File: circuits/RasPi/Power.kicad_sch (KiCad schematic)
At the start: 84 parts, among them J4 Conn_01x02_Pin, Q11 2N7002, Q12 SSM6J808R, Q14 SSM6J808R, Q15 S8550, Q16 SSM6J808R, Q17 S8550, Q6 SSM3J332R, Q7 S8550, Q8 SSM3J332R, Q9 S8550, SW4 SW_SPDT, U13 TPS54560BDDA, U16 AZ1117CH-3.3, U17 M51957B, U19 DCDC_TPS61023

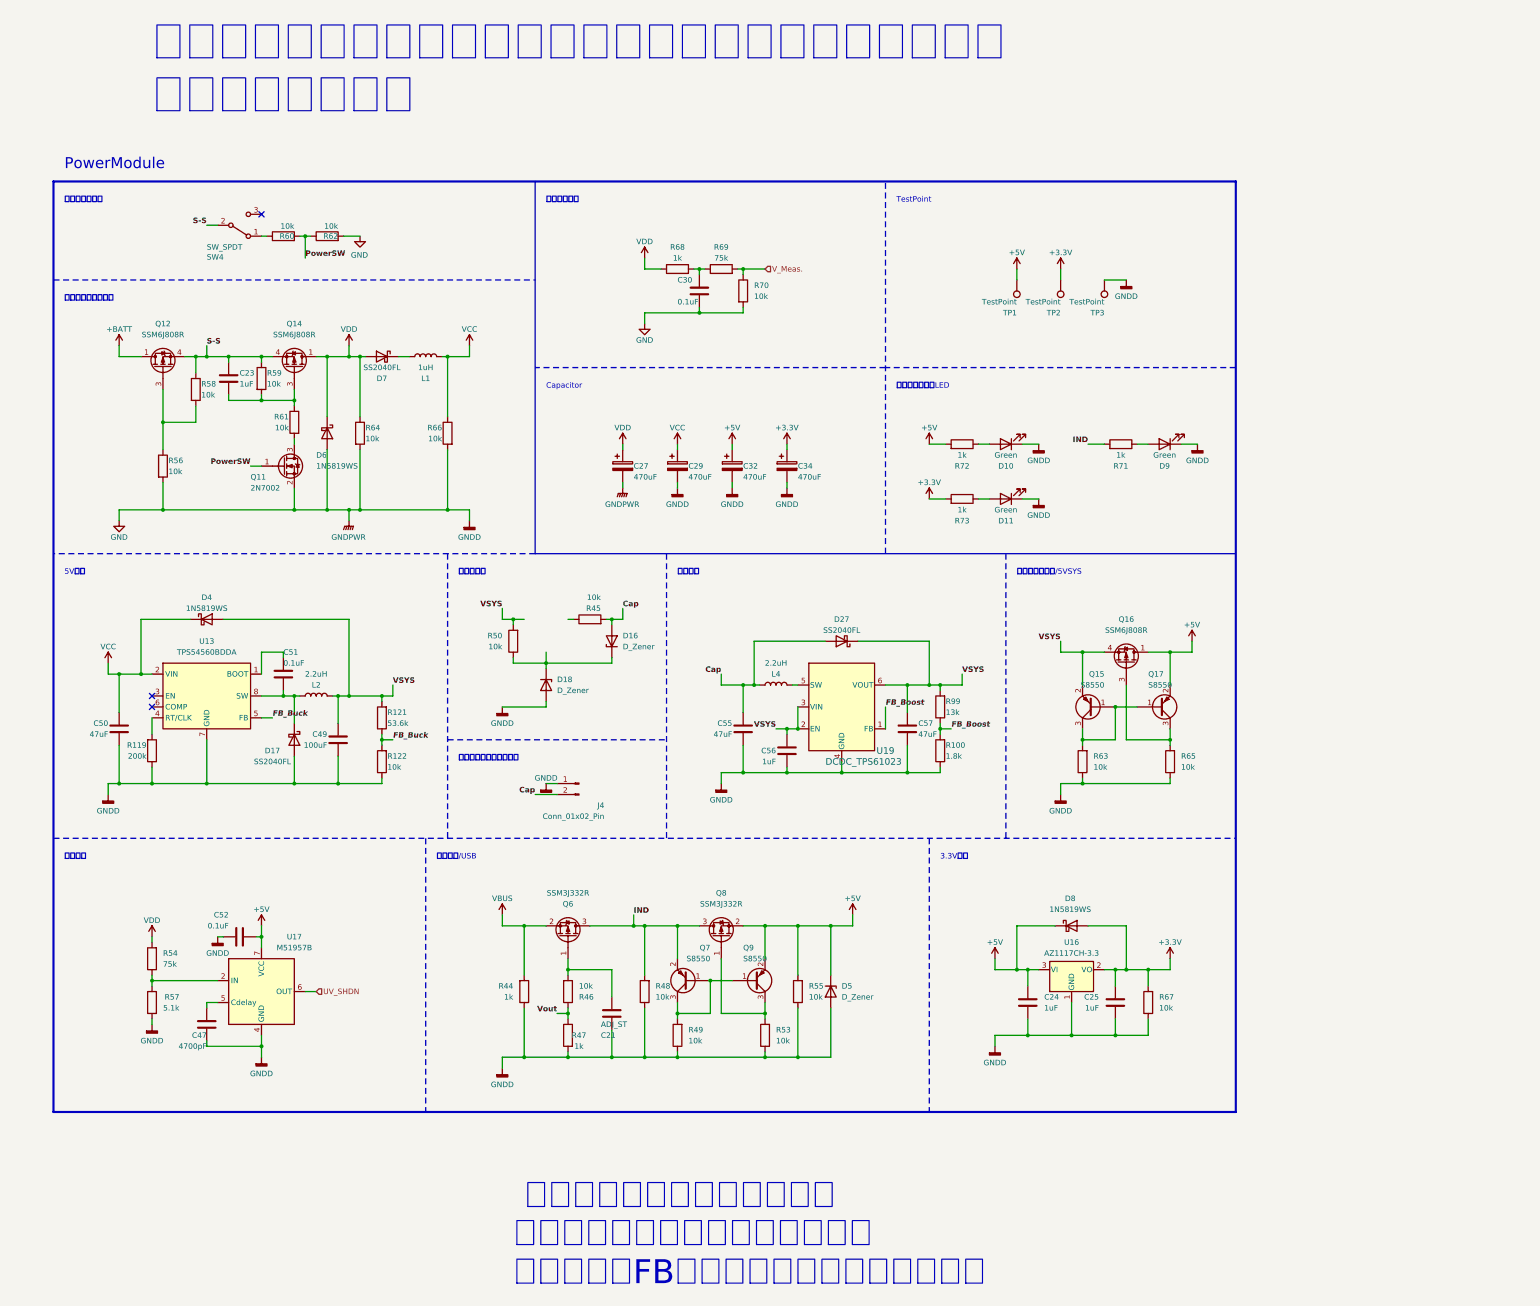
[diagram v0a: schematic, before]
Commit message: raspi基板回路図
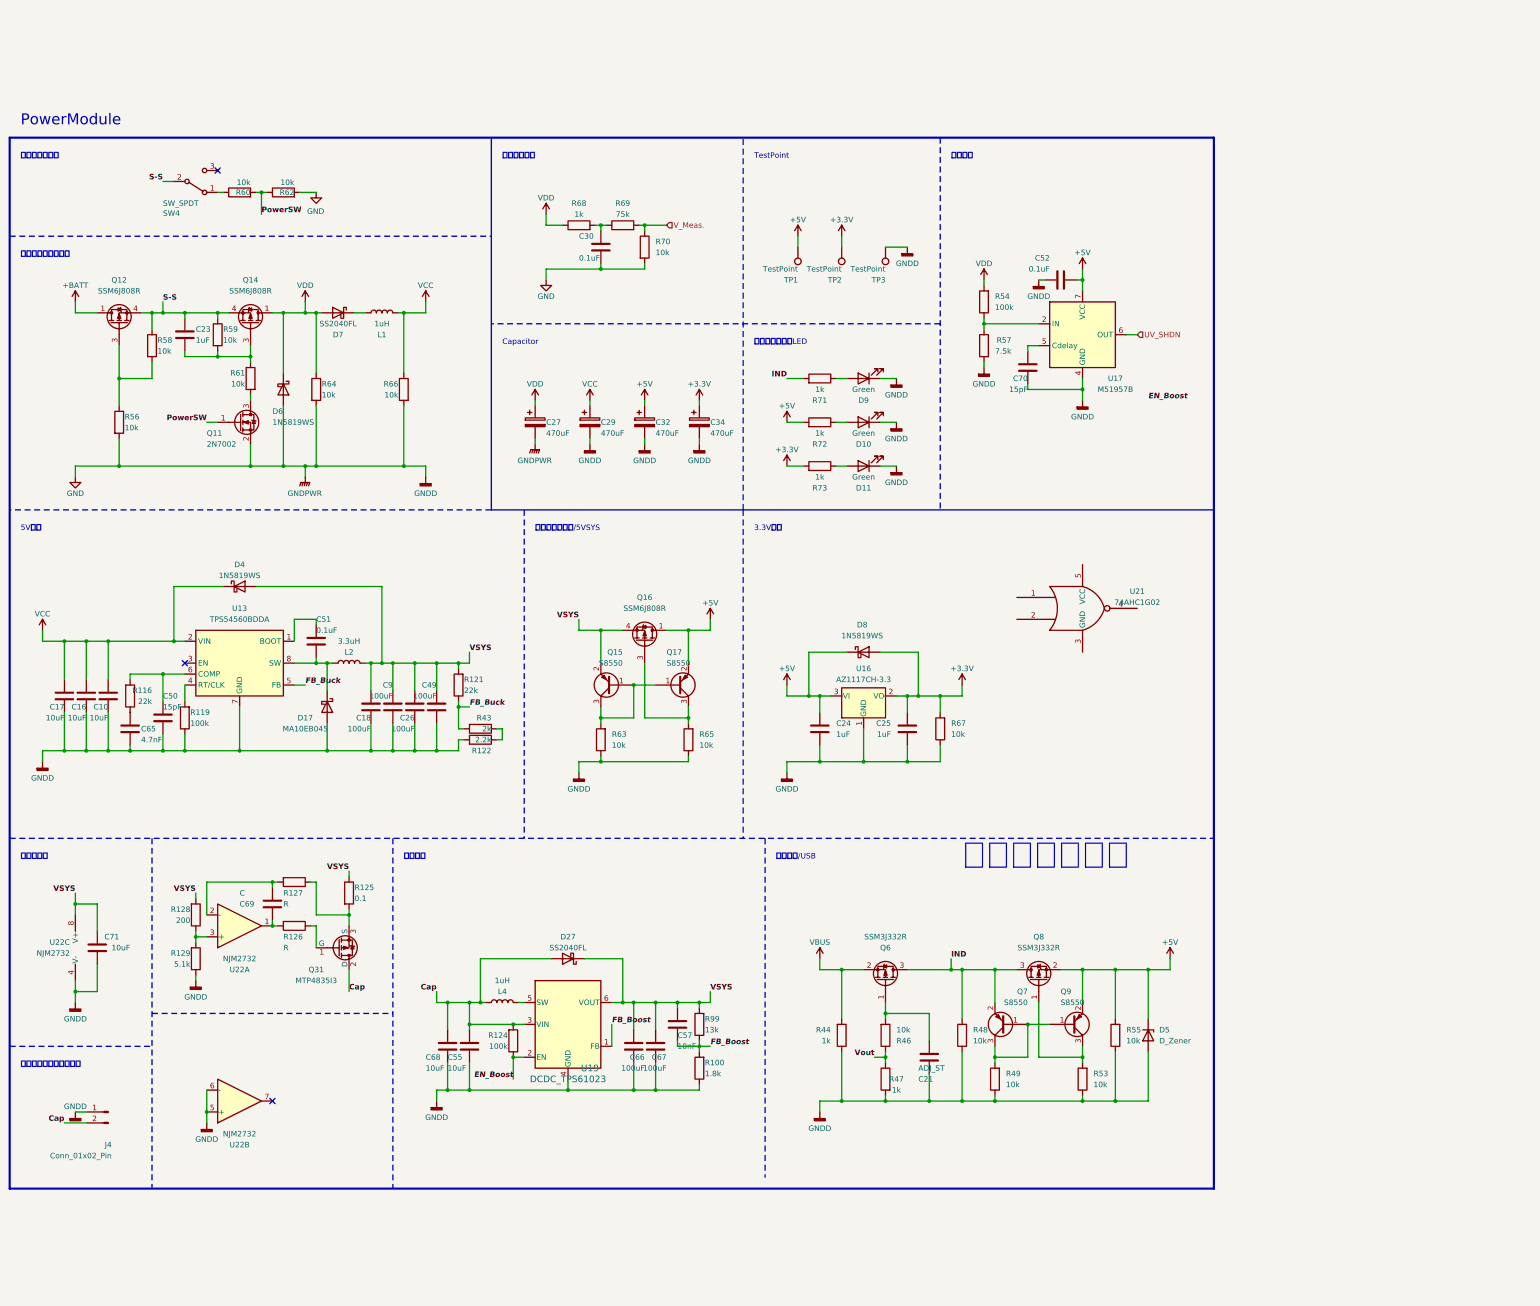
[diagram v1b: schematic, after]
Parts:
- removed C47: 4700pF, Capacitor_SMD:C_0603_1608Metric, symbol Device:C
- removed C56: 1uF, Capacitor_SMD:C_0603_1608Metric, symbol Device:C
- removed D16, D18: D_Zener, Diode_SMD:D_SOD-323_HandSoldering, symbol Device:D_Zener
- removed R45, R50: 10k, Resistor_SMD:R_0402_1005Metric, symbol Device:R
- added C10, C16, C17: 10uF, Capacitor_SMD:C_1206_3216Metric, symbol Device:C
- added C18, C26, C66, C67, C9: 100uF, Capacitor_SMD:C_1206_3216Metric, symbol Device:C
- added C65: 4.7nF, Capacitor_SMD:C_0402_1005Metric, symbol Device:C
- added C68, C71: 10uF, Capacitor_SMD:C_0805_2012Metric, symbol Device:C
- added C69: C, Resistor_SMD:R_0603_1608Metric, symbol Device:C
- added C70: 15pF, Capacitor_SMD:C_0402_1005Metric, symbol Device:C
- added Q31: MTP4835I3, Package_TO_SOT_SMD:TO-252-2, symbol Device:Q_PMOS_GDS
- added R116: 22k, Resistor_SMD:R_0402_1005Metric, symbol Device:R
- added R124: 100k, Resistor_SMD:R_0402_1005Metric, symbol Device:R
- added R125: 0.1, symbol Device:R
- added R126, R127: R, Resistor_SMD:R_0603_1608Metric, symbol Device:R
- added R128: 200, Resistor_SMD:R_0402_1005Metric, symbol Device:R
- added R129: 5.1k, Resistor_SMD:R_0402_1005Metric, symbol Device:R
- added R43: 2k, Resistor_SMD:R_0402_1005Metric, symbol Device:R
- added U21: 74AHC1G02, Package_TO_SOT_SMD:SOT-23-5, symbol 74xGxx:74AHC1G02
- added U22: NJM2732, symbol Amplifier_Operational:LM7332
- C49: footprint Capacitor_SMD:C_0805_2012Metric -> Capacitor_SMD:C_1206_3216Metric
- C50: value 47uF -> 15pF; footprint Capacitor_SMD:C_0805_2012Metric -> Capacitor_SMD:C_0402_1005Metric
- C51: footprint Capacitor_SMD:C_0603_1608Metric -> Capacitor_SMD:C_0402_1005Metric
- C55: value 47uF -> 10uF
- C57: value 47uF -> 10nF; footprint Capacitor_SMD:C_0805_2012Metric -> Capacitor_SMD:C_0402_1005Metric
- D17: value SS2040FL -> MA10EB045; footprint Diode_SMD:D_SOD-123 -> Diode_SMD:Vishay_SMPA
- L2: value 2.2uH -> 3.3uH; footprint (none) -> TomoshibiLibrary:Inductor_ECS-MPIL0530
- L4: value 2.2uH -> 1uH; footprint (none) -> Inductor_SMD:L_1210_3225Metric
- R119: value 200k -> 100k
- R121: value 53.6k -> 22k
- R122: value 10k -> 2.2k
- R54: value 75k -> 100k
- R57: value 5.1k -> 7.5k
- SW4: footprint TomoshibiLibrary:SW_Slide_SPDT_White -> TomoshibiLibrary:SW_Slide_SPDT_IS-1235-G
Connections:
- net Cap: now also C55.2, U19.3 (VIN), C68.2, Q31.2 (D), R124.2; no longer C55.1
- net FB_Boost: now also C57.2
- net FB_Buck: now also R43.2; no longer R122.2
- net GND: now also C55.1, R122.2, C10.2, C16.2, C17.2, C18.2, C26.2, C65.2, C66.2, C67.2, C68.1, C70.2, C71.1, C9.2, R129.1, U22.4 (V-), U22.5 (+), U22.6 (-); no longer C55.2, C57.2, R122.1
- net VCC: now also C10.1, C16.1, C17.1; no longer C50.1
- net VSYS: now also C18.1, C26.1, C66.1, C67.1, C71.2, C9.1, R125.1, R128.2, U22.8 (V+); no longer U19.2 (EN), U19.3 (VIN)
- net at U17.5 (Cdelay): now also C70.1
- net at U13.6 (COMP): now also C50.1, R116.2
- new net: C65.1, R116.1
- new net: C69.1, R126.2, U22.1
- new net: C69.2, R127.2, U22.2 (-)
- new net: R128.1, R129.2, U22.3 (+)
- new net: Q31.1 (G), R126.1
- new net: Q31.3 (S), R125.2, R127.1
- new net: R122.1, R43.1
- new net EN_Boost: R124.1, U19.2 (EN)
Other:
- note added: "ダイオード変更"
- note removed: "スライドスイッチの色分けとか、スイッチの区別を見直す 電源は白スライド"
- note removed: "三端子を新しく選定したのにする 昇圧回路のFB電圧をちょっと低く設定する"
- note removed: "電源スイッチ 耐圧大丈夫？"
- moved on the sheet: C21, C23, C24, C25, C27, C29, C30, C32, C34, C51, C52, D10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
